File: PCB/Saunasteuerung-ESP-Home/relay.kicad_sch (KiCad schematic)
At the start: 43 parts, among them J1 HB9500M-9.5-6P, J2 HB9500M-9.5-6P, J3 HB9500M-9.5-6P, J4 HB9500M-9.5-3P, K1 RAYEX-L90, K2 RAYEX-L90, K3 RAYEX-L90, K4 SANYOU_SRD_Form_C, K5 SANYOU_SRD_Form_C, Q1 S8550, Q2 S8550, Q3 S8550, Q5 2N222, Q6 2N222, U1 FODM217A, U2 FODM217A, U3 FODM217A

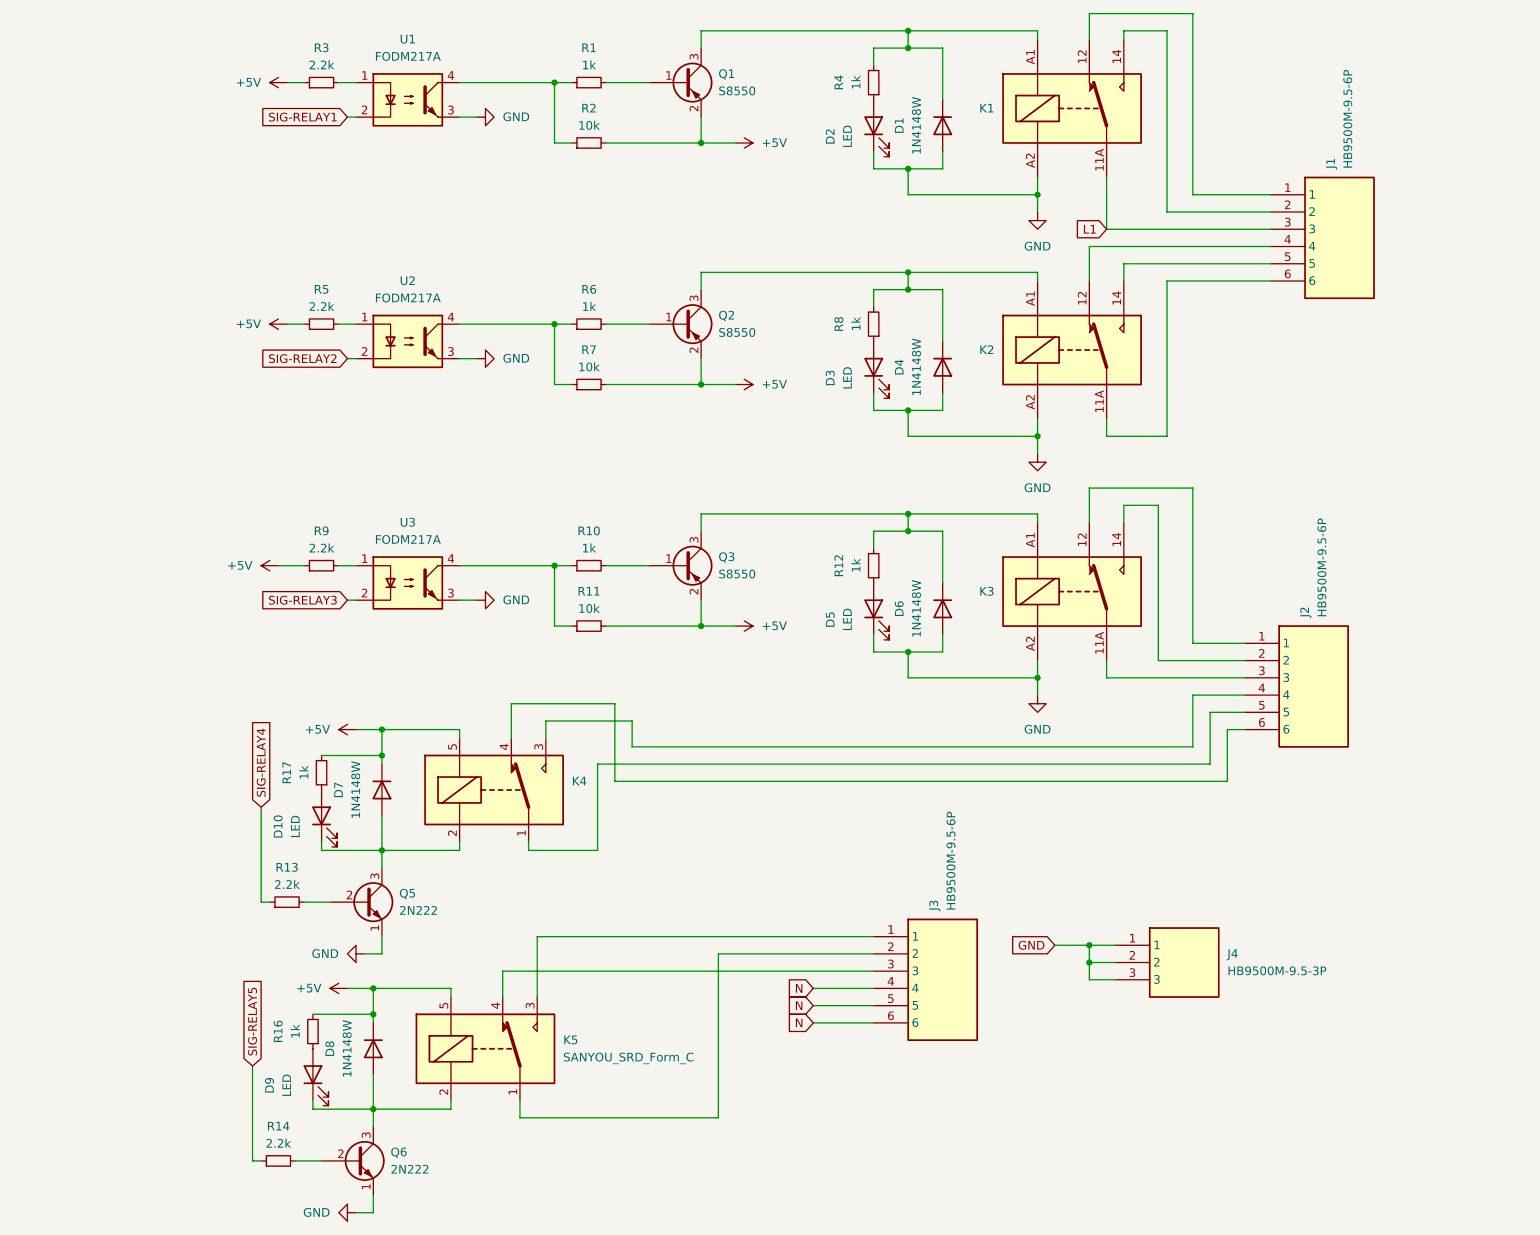
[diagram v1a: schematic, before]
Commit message: V2.0 push
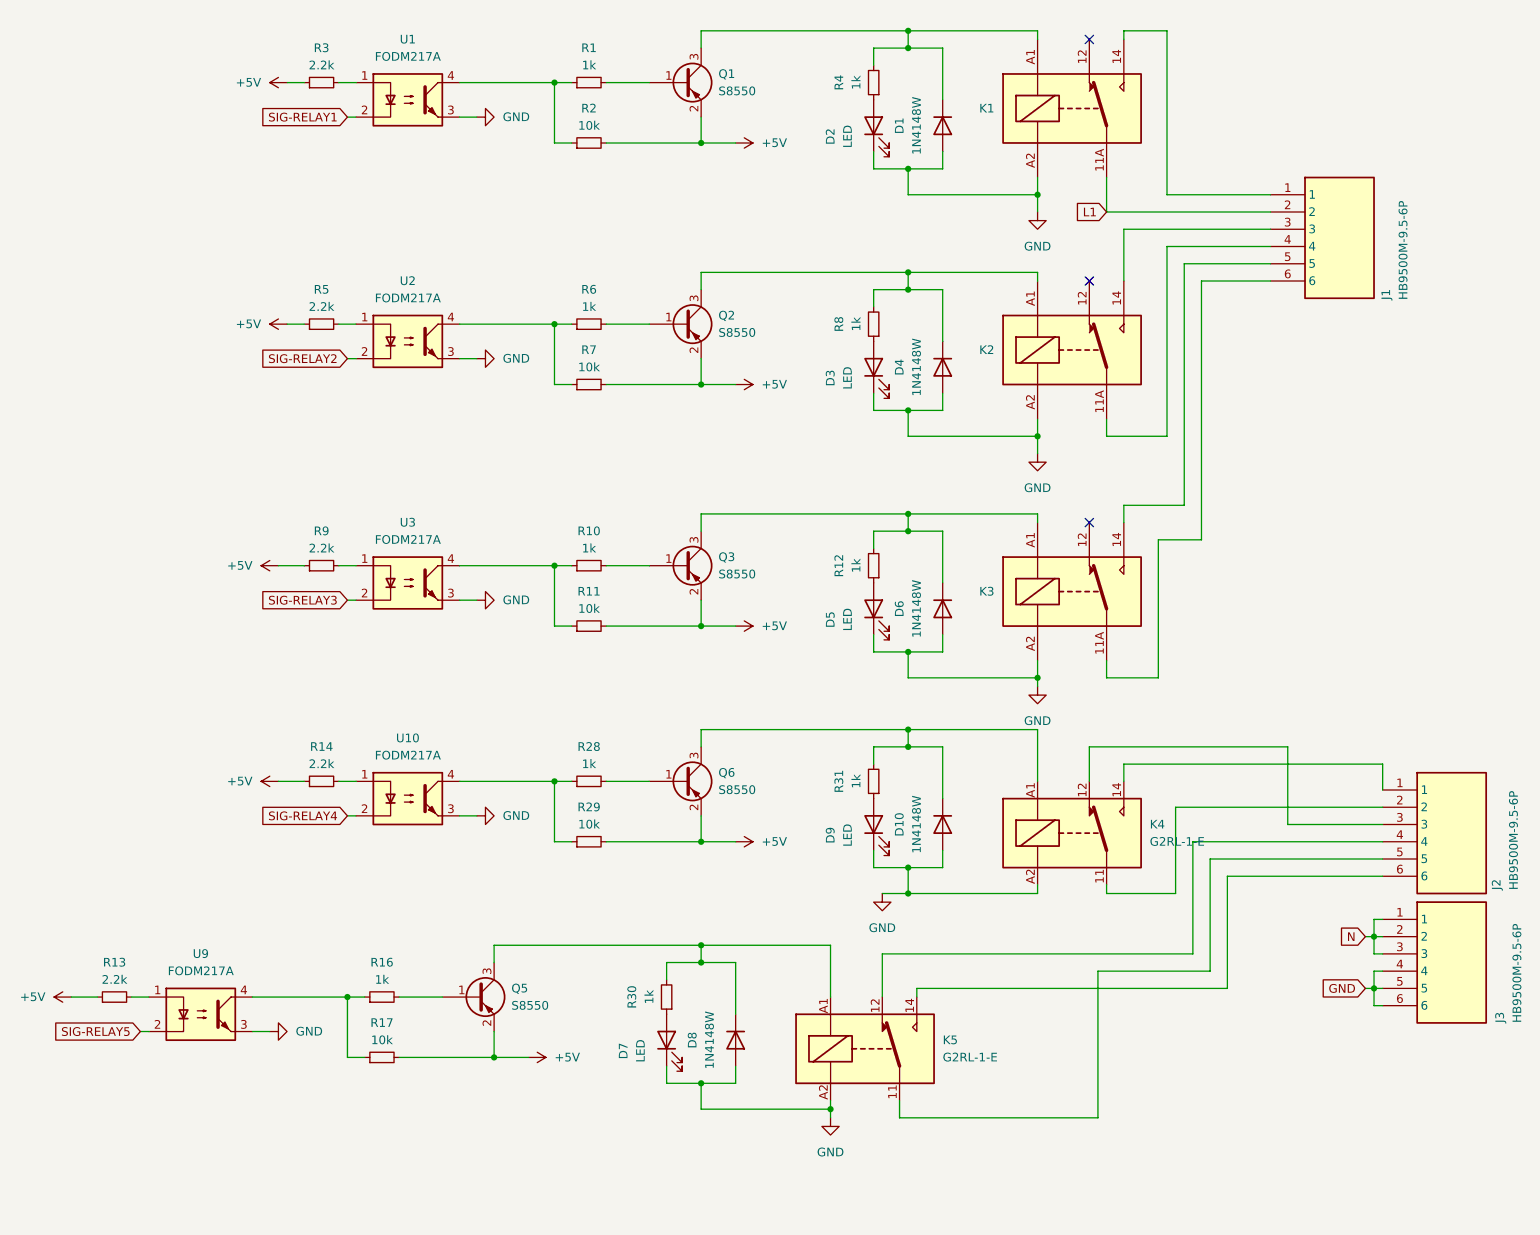
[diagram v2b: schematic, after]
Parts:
- removed D10: LED, LED_SMD:LED_0603_1608Metric, symbol Device:LED
- removed D7: 1N4148W, Diode_SMD:D_SOD-123, symbol Diode:1N4148W
- removed J4: HB9500M-9.5-3P, Samacsys:HB9500M953P, symbol Samacsys:HB9500M-9.5-3P
- removed K4, K5: SANYOU_SRD_Form_C, Relay_THT:Relay_SPDT_SANYOU_SRD_Series_Form_C, symbol Relay:SANYOU_SRD_Form_C
- removed Q5, Q6: 2N222, Package_TO_SOT_THT:TO-92L, symbol Transistor_BJT:2N3904
- added D10: 1N4148W, Diode_SMD:D_SOD-123, symbol Diode:1N4148W
- added D7: LED, LED_SMD:LED_0603_1608Metric, symbol Device:LED
- added K4, K5: G2RL-1-E, Relay_THT:Relay_SPDT_Omron_G2RL-1-E, symbol Relay:G2RL-1-E
- added Q5, Q6: S8550, Package_TO_SOT_SMD:SOT-23, symbol Transistor_BJT:BC807
- added R28, R30, R31: 1k, Resistor_SMD:R_0603_1608Metric, symbol Device:R_Small
- added R29: 10k, Resistor_SMD:R_0603_1608Metric, symbol Device:R_Small
- added U10, U9: FODM217A, Package_SO:SOP-4_4.4x2.6mm_P1.27mm, symbol Isolator:FODM217A
- R17: value 1k -> 10k
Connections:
- net +5V: now also R13.1, R14.1, Q5.2 (E), Q6.2 (E), R29.2; no longer D8.1 (K), R16.2
- net GND: now also D8.2 (A), D9.1 (K), J3.4, J3.5, J3.6, D10.2 (A), D7.1 (K), K4.A2, K5.A2, U10.3, U9.3
- net L1: now also J1.2; no longer J1.3
- net N: now also J3.1, J3.2, J3.3; no longer J3.4, J3.5, J3.6
- net SIG-RELAY4: now also U10.2; no longer R13.1
- net SIG-RELAY5: now also U9.2; no longer R14.1
- net at D9.2 (A): now also R31.1; no longer R16.1
- net at R17.1: now also R16.1, U9.4
- net at J2.1: now also K4.14; no longer K3.12
- net at J2.2: now also K4.11; no longer K3.14
- net at K3.11A, K3.11B: now also J1.6; no longer J2.3
- net at J2.4: now also K5.12
- net at J2.5: now also K5.11
- net at J2.6: now also K5.14
- net at R13.2: now also U9.1
- net at J1.1: now also K1.14; no longer K1.12
- net at J1.4: now also K2.11A, K2.11B; no longer K2.12
- net at K2.14: now also J1.3; no longer J1.5
- net at R14.2: now also U10.1
- new net: D8.1 (K), K5.A1, Q5.3 (C), R30.2
- new net: J2.3, K4.12
- new net: D10.1 (K), K4.A1, Q6.3 (C), R31.2
- new net: R28.1, R29.1, U10.4
- new net: Q6.1 (B), R28.2
- new net: J1.5, K3.14
- new net: Q5.1 (B), R16.2
- new net: D7.2 (A), R30.1
- no-connect marks 0 -> 3
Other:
- moved on the sheet: J2, J3
